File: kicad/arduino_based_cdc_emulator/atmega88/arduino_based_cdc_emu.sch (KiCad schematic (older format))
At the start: 15 parts, among them IC1 ATMEGA88-A, P1 CONN_1, P2 CONN_2, P3 CONN_3, U1 78L05, X1 20MHz

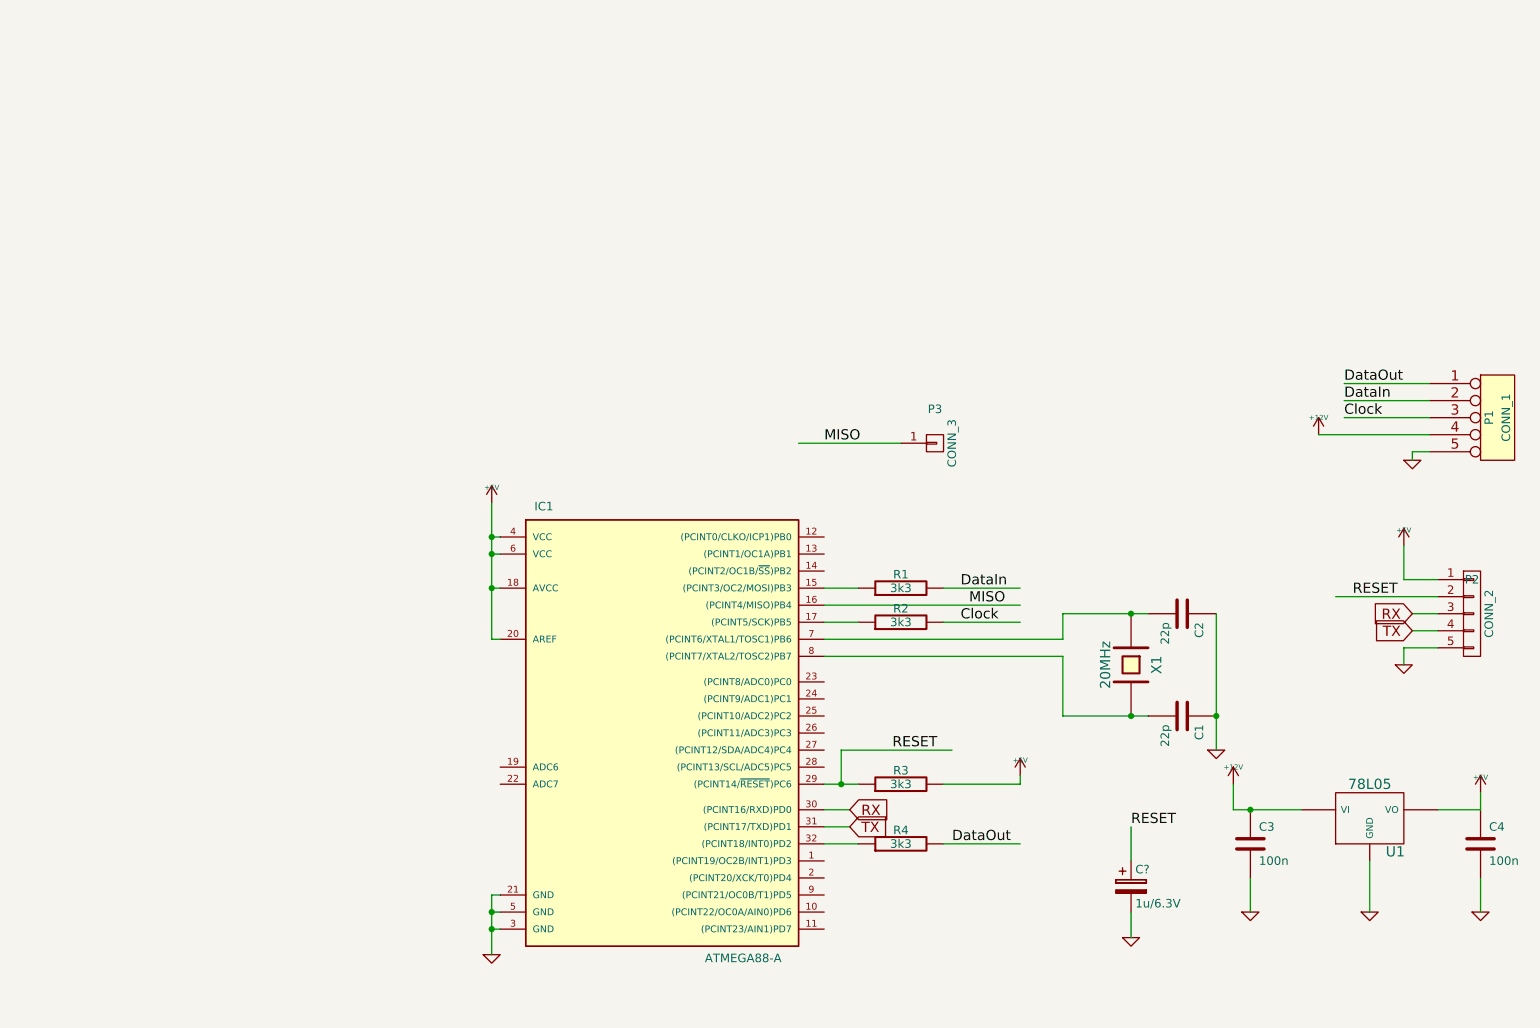
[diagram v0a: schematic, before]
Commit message: update
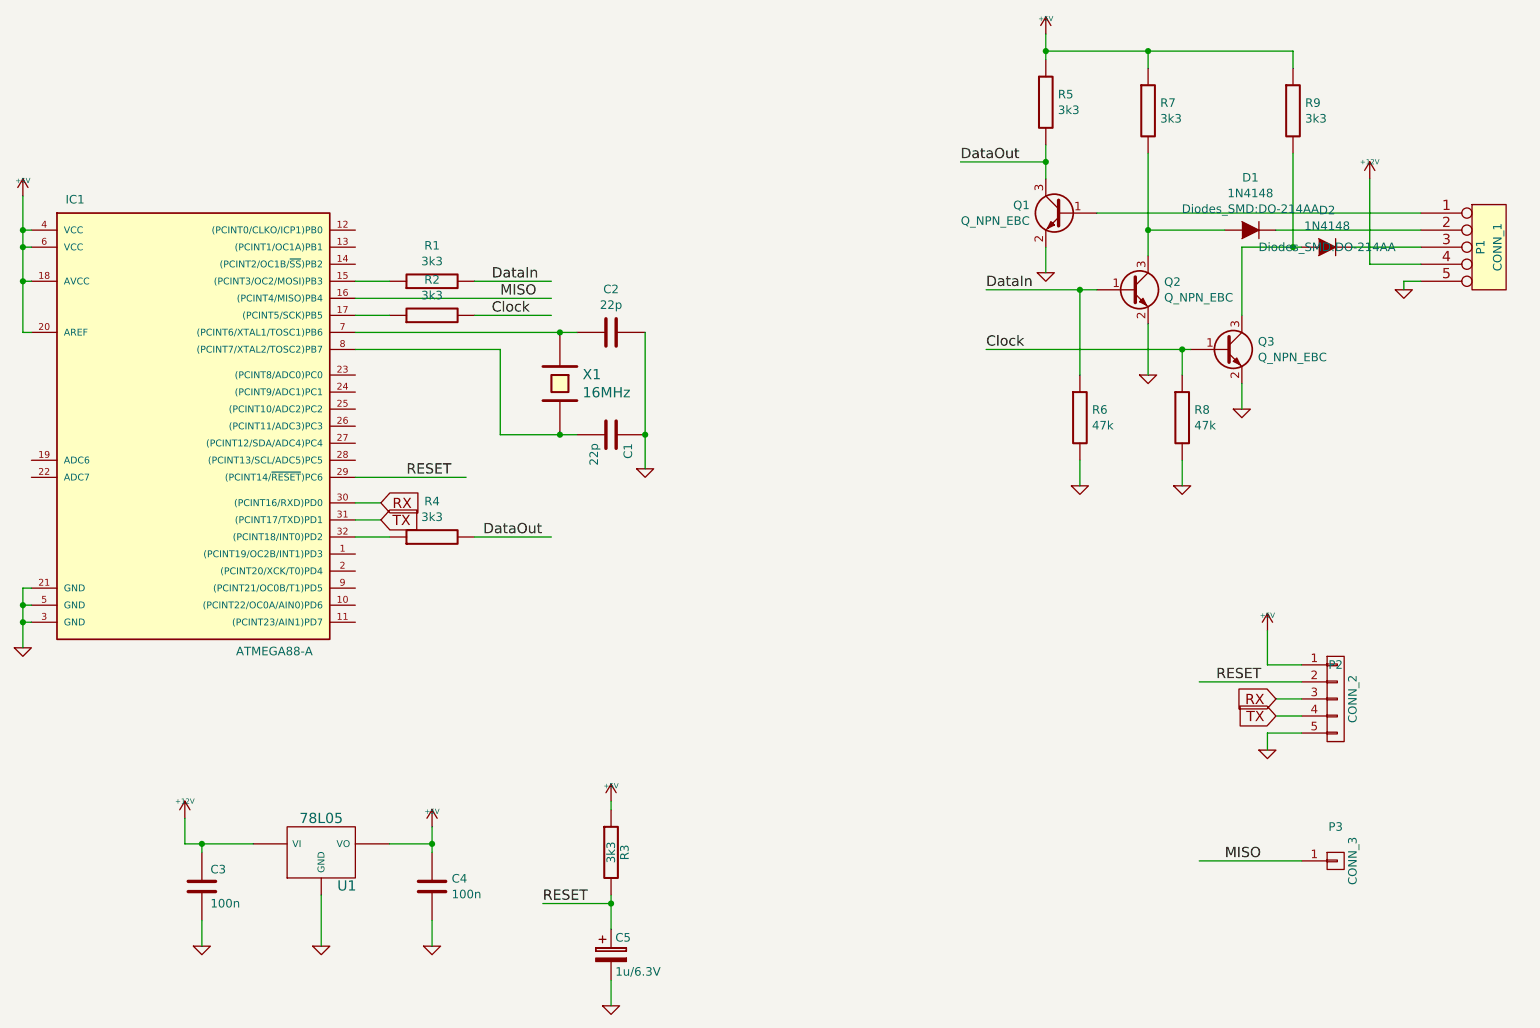
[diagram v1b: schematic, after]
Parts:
- added D1, D2: 1N4148, Diodes_SMD:DO-214AA, symbol D
- added Q1, Q2, Q3: Q_NPN_EBC, symbol Q_NPN_BEC
- added R5, R7, R9: 3k3, Resistors_SMD:R_0805_HandSoldering, symbol R-RESCUE-arduino_based_cdc_emu
- added R6, R8: 47k, Resistors_SMD:R_0805_HandSoldering, symbol R-RESCUE-arduino_based_cdc_emu
- C1, C2: footprint Capacitors_SMD:C_1206_HandSoldering -> Capacitors_SMD:C_0805
- C3, C4: footprint Capacitors_SMD:C_1206_HandSoldering -> Capacitors_SMD:C_0805_HandSoldering
- R1, R2, R4: footprint Resistors_SMD:R_1206_HandSoldering -> Resistors_SMD:R_0805
- R3: footprint Resistors_SMD:R_1206_HandSoldering -> Resistors_SMD:R_0805_HandSoldering
- X1: value 20MHz -> 16MHz
- gave numbers to parts that had none: 1
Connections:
- wire segments 53 -> 71
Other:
- moved on the sheet: C1, C2, C3, C4, C5, IC1, P1, P2, P3, R1, R2, R3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
